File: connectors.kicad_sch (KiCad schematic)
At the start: 20 parts, among them J5V1 Conn_01x02, J5V10 Conn_01x02, J5V11 Conn_01x02, J5V12 Conn_01x02, J5V13 Conn_01x02, J5V14 Conn_01x02, J5V15 Conn_01x02, J5V16 Conn_01x02, J5V17 Conn_01x02, J5V18 Conn_01x02, J5V19 Conn_01x02, J5V2 Conn_01x02, J5V20 Conn_01x02, J5V3 Conn_01x02, J5V4 Conn_01x02, J5V5 Conn_01x02, J5V6 Conn_01x02, J5V7 Conn_01x02, J5V8 Conn_01x02, J5V9 Conn_01x02

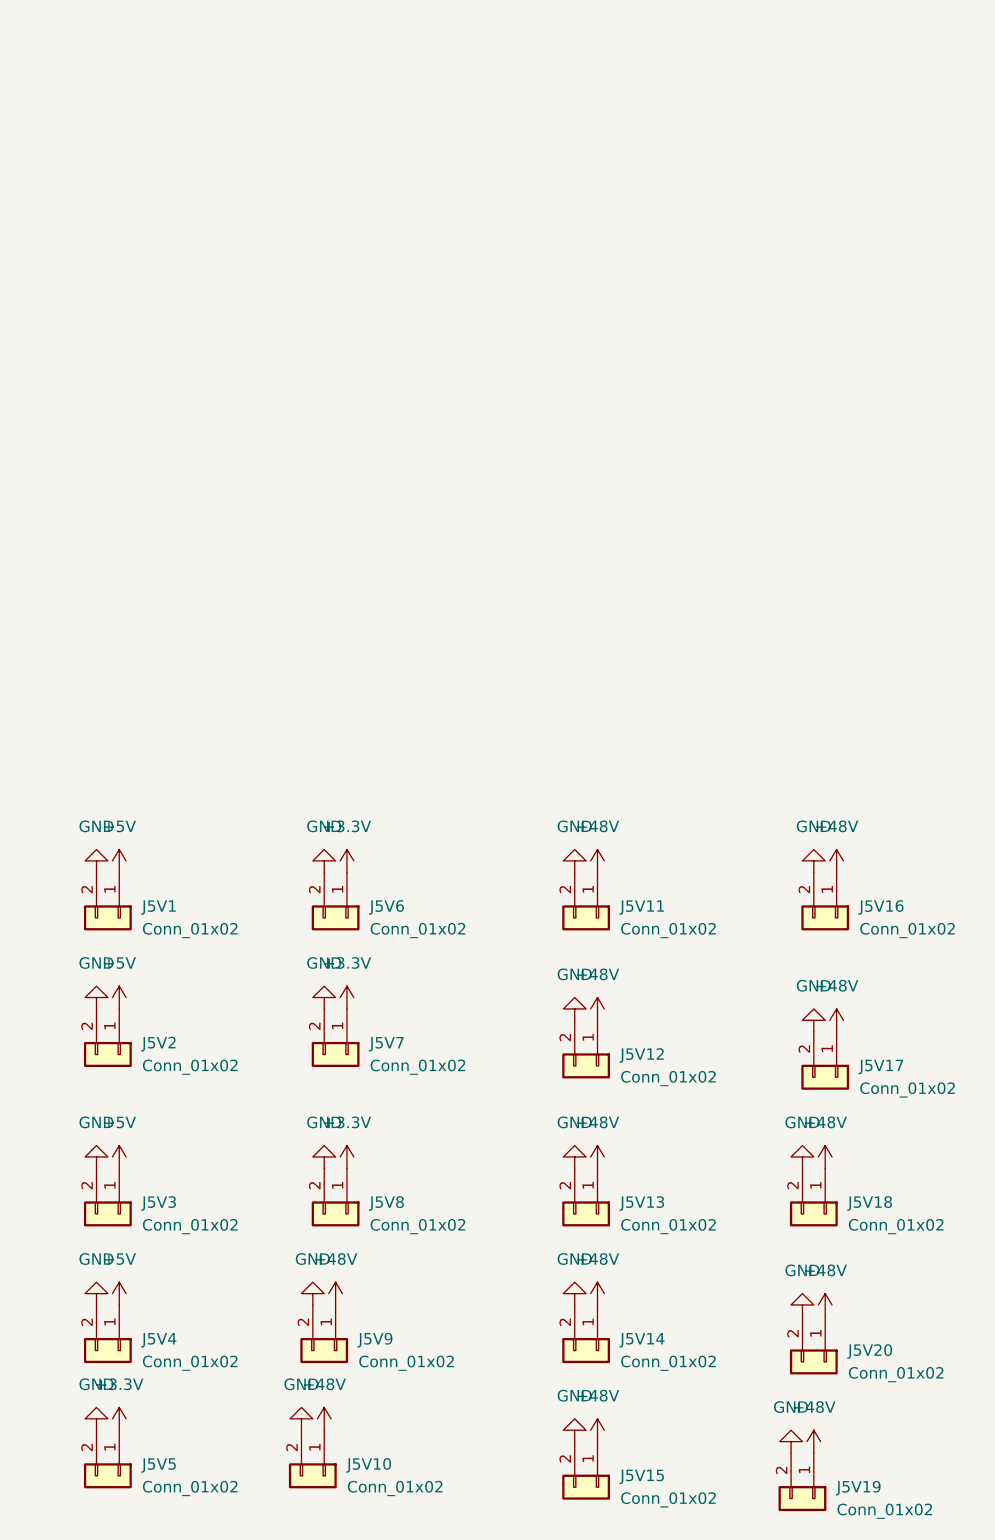
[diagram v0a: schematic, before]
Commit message: updates
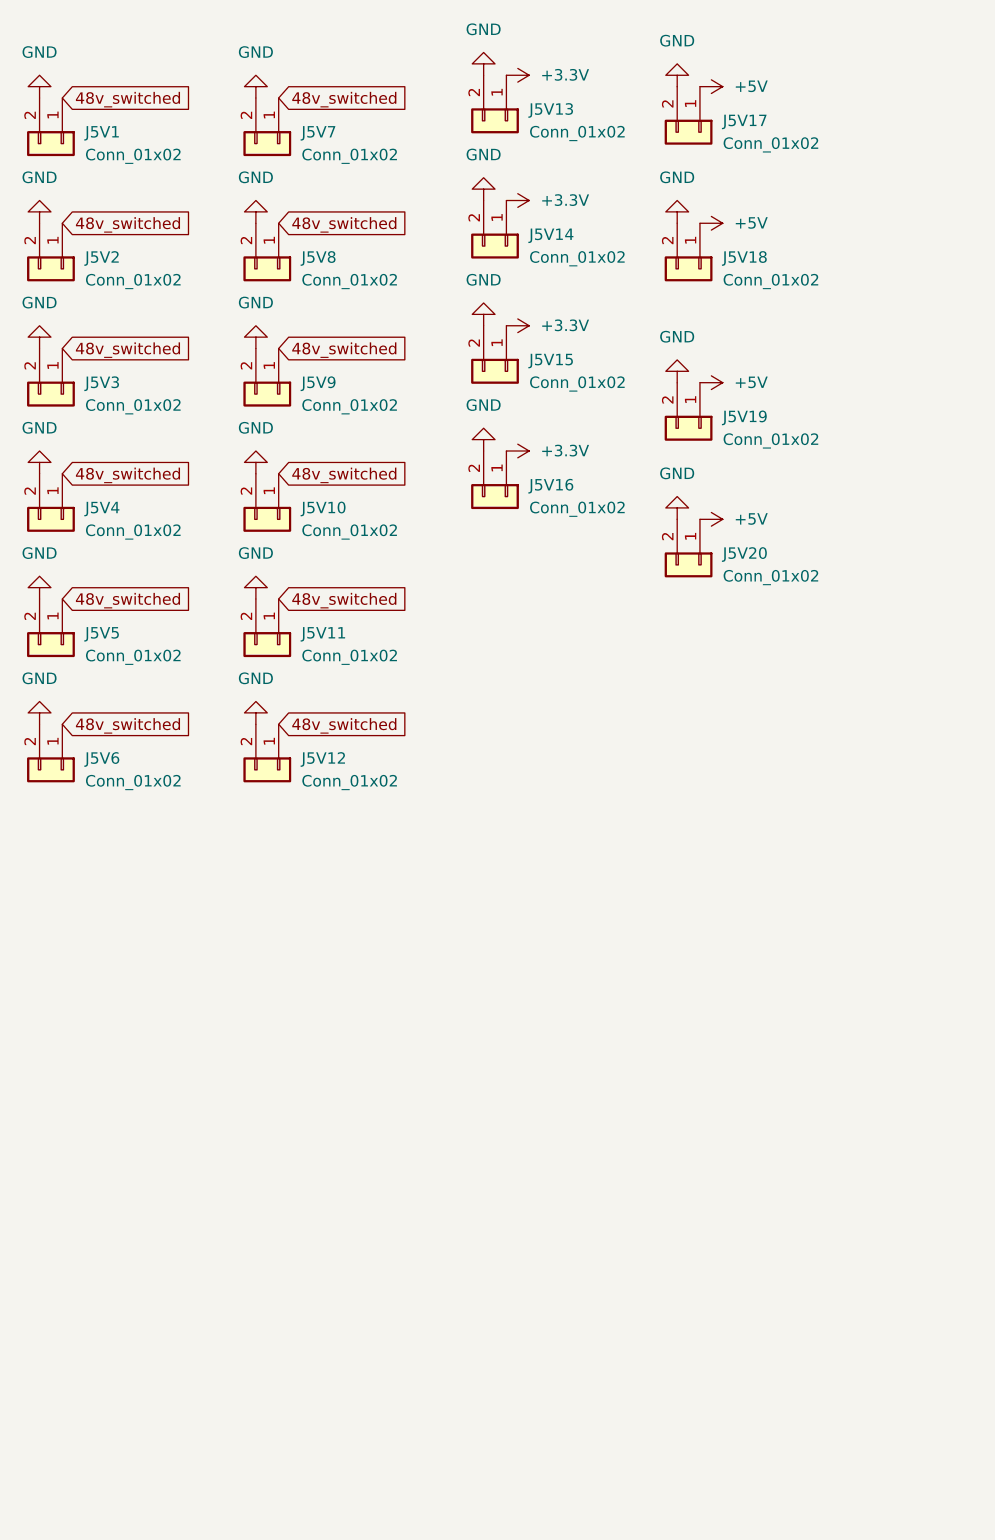
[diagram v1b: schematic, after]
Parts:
- removed J5V10, J5V11, J5V13, J5V14: Conn_01x02, Connector_AMASS:AMASS_XT30PW-F_1x02_P2.50mm_Horizontal, symbol Connector_Generic:Conn_01x02
- added J5V4, J5V5, J5V7, J5V8: Conn_01x02, Connector_AMASS:AMASS_XT30U-F_1x02_P5.0mm_Vertical, symbol Connector_Generic:Conn_01x02
- J5V12, J5V9: footprint Connector_AMASS:AMASS_XT30PW-F_1x02_P2.50mm_Horizontal -> Connector_AMASS:AMASS_XT30U-F_1x02_P5.0mm_Vertical
- renumbered J5V16 to J5V1, J5V20 to J5V10, J5V19 to J5V11, J5V6 to J5V13, J5V7 to J5V14, J5V8 to J5V15, J5V5 to J5V16, J5V1 to J5V17, J5V2 to J5V18, J5V3 to J5V19, J5V17 to J5V2, J5V4 to J5V20, J5V18 to J5V3, J5V15 to J5V6
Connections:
- net GND: now also J5V4.2 (Pin_2), J5V5.2 (Pin_2), J5V7.2 (Pin_2), J5V8.2 (Pin_2)
- net +48V renamed 48v_switched
- net 48v_switched: now also J5V4.1 (Pin_1), J5V5.1 (Pin_1), J5V7.1 (Pin_1), J5V8.1 (Pin_1)
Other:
- moved on the sheet: J5V1, J5V10, J5V11, J5V13, J5V14, J5V15, J5V16, J5V17, J5V18, J5V19, J5V2, J5V20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
